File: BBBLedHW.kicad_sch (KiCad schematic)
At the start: 40 parts, among them J3 Barrel_Jack_Switch, Q1 2N7002, U1 STM32WB55CEUx, U2 TPS7A2033DBV, U3 SN74LVC1T45DBV, U4 ADP2303ARDZ-5.0, X1 32MHz, X2 32kHz768

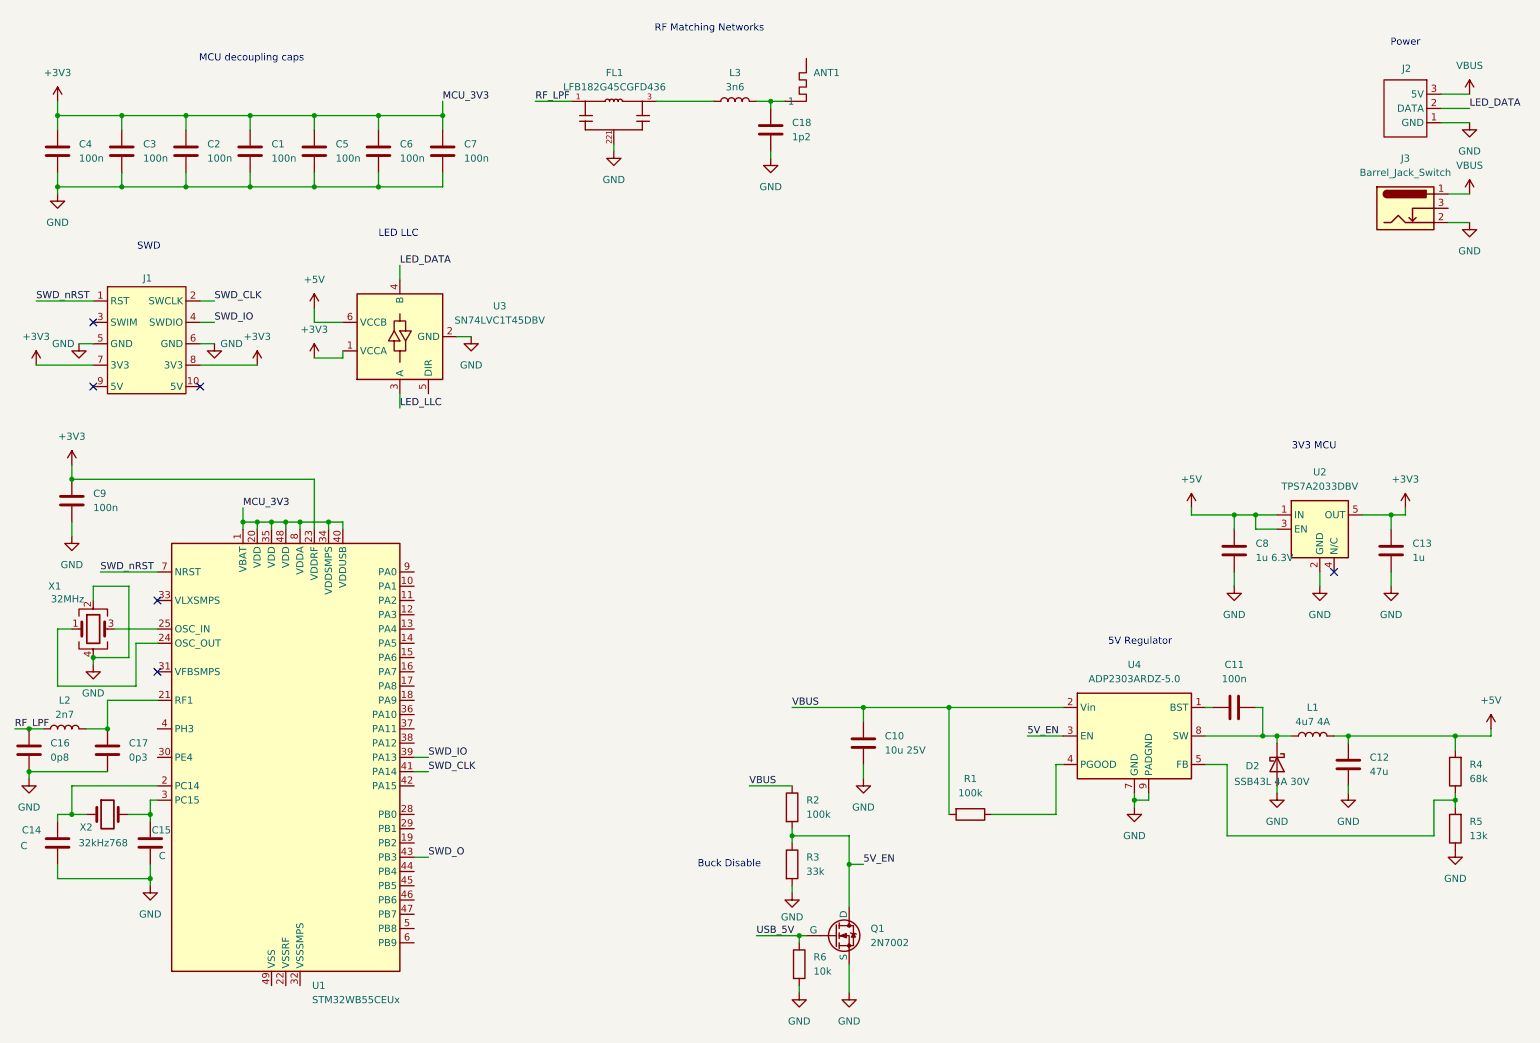
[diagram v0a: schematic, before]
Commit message: Final touches before review
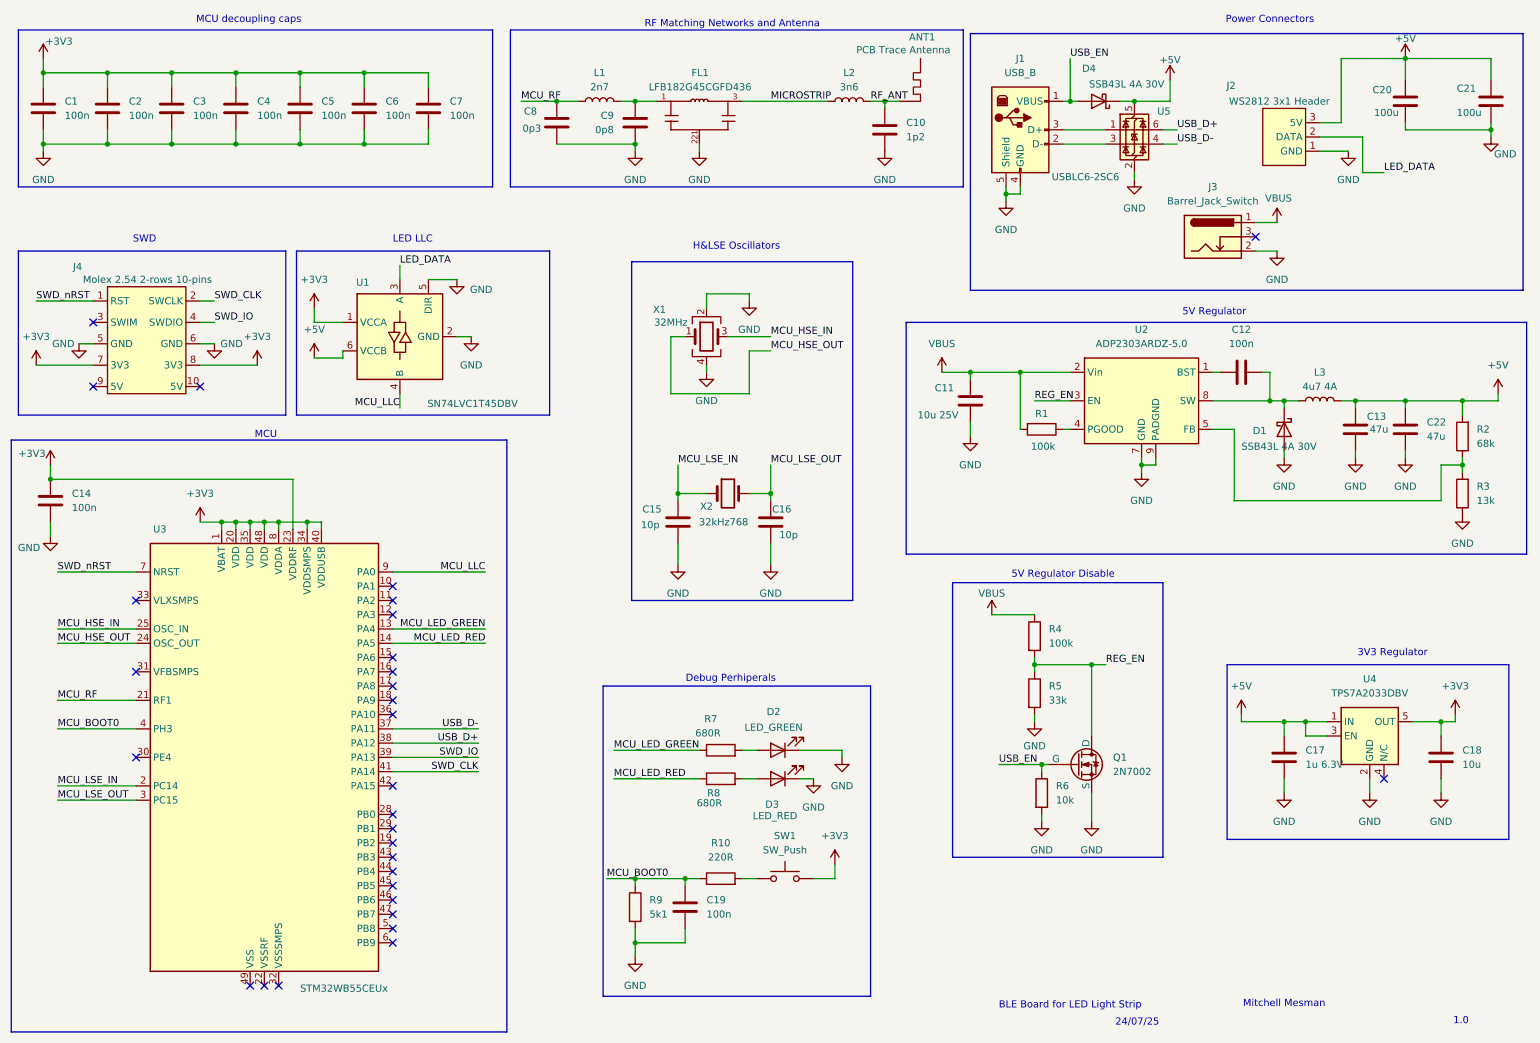
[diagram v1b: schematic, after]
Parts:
- added C19: 100n, symbol Device:C
- added C20, C21: 100u, symbol Device:C
- added C22: 47u, symbol Device:C
- added D2: LED_GREEN, symbol Device:LED
- added D3: LED_RED, symbol Device:LED
- added D4: SSB43L 4A 30V, symbol Device:D_Schottky
- added J1: USB_B, symbol Connector:USB_B
- added R10: 220R, symbol Device:R
- added R7, R8: 680R, symbol Device:R
- added R9: 5k1, symbol Device:R
- added SW1: SW_Push, symbol Switch:SW_Push
- added U5: USBLC6-2SC6, Package_TO_SOT_SMD:SOT-23-6, symbol Power_Protection:USBLC6-2SC6
- ANT1: value ~ -> PCB Trace Antenna
- C15: renamed from C14; value C -> 10p
- C16: renamed from C15; value C -> 10p
- C18: renamed from C13; value 1u -> 10u
- J2: value ~ -> WS2812 3x1 Header
- J4: renamed from J1; value ~ -> Molex 2.54 2-rows 10-pins
- renumbered C4 to C1, C18 to C10, C10 to C11, C11 to C12, C12 to C13, C9 to C14, C8 to C17, C3 to C2, C2 to C3, C1 to C4, C17 to C8, C16 to C9, D2 to D1, L2 to L1, L3 to L2, L1 to L3, R4 to R2, R5 to R3, R2 to R4, R3 to R5, U3 to U1, U4 to U2, U1 to U3, U2 to U4
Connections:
- net LED_LLC is gone; now on net LED_DATA: U1.3 (A)
- net +3V3: now also SW1.2
- net +5V: now also J2.3 (5V), C20.1, C21.1, C22.1, D4.1 (K), U5.5 (VBUS)
- net GND: now also U1.5 (DIR), C19.2, C20.2, C21.2, C22.2, D2.1 (K), D3.1 (K), J1.4 (GND), J1.5 (Shield), R9.2, U5.2 (GND)
- net LED_DATA: no longer U1.4 (B)
- net VBUS: no longer J2.3 (5V)
- net MCU_LSE_OUT: now reaches C16.1, U3.3 (PC15), X2.2
- net MCU_LED_GREEN: now reaches U3.13 (PA4)
- net MCU_LED_GREEN: now also R7.1
- net MCU_LED_RED: now reaches U3.14 (PA5)
- net MCU_LED_RED: now also R8.1
- net MCU_LSE_IN: now reaches C15.1, U3.2 (PC14), X2.1
- net MCU_RF: now reaches C8.1, L1.2, U3.21 (RF1)
- net MCU_HSE_OUT: now reaches U3.24 (OSC_OUT), X1.1
- net MCU_HSE_IN: now reaches U3.25 (OSC_IN), X1.3
- net USB_D-: now reaches U3.37 (PA11)
- net USB_D-: now also U5.4 (I/O2)
- net USB_D+: now reaches U3.38 (PA12)
- net USB_D+: now also U5.6 (I/O1)
- net MCU_BOOT0: now reaches U3.4 (PH3)
- net MCU_BOOT0: now also C19.1, R10.1, R9.1
- net MCU_LLC: now reaches U3.9 (PA0)
- net MCU_LLC: now also U1.4 (B)
- net MICROSTRIP: now reaches FL1.3, L2.1
- net RF_ANT: now reaches ANT1., C10.1, L2.2
- net 5V_EN renamed REG_EN
- net RF_LPF: no longer names the net of C9.1, FL1.1, L1.1
- net SWD_O: no longer names the net of U3.43 (PB3)
- net USB_5V renamed USB_EN
- net USB_EN: now also D4.2 (A), J1.1 (VBUS)
- new net: D2.2 (A), R7.2
- new net: J1.3 (D+), U5.1 (I/O1)
- new net: J1.2 (D-), U5.3 (I/O2)
- new net: D3.2 (A), R8.2
- new net: R10.2, SW1.1
- no-connect marks 6 -> 30
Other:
- note added: "1.0"
- note added: "24/07/25"
- note added: "3V3 Regulator"
- note added: "5V Regulator Disable"
- note added: "BLE Board for LED Light Strip"
- note added: "Debug Perhiperals"
- note added: "H&LSE Oscillators"
- note added: "MCU"
- note added: "Mitchell Mesman"
- note added: "Power Connectors"
- note added: "RF Matching Networks and Antenna"
- note removed: "3V3 MCU"
- note removed: "Buck Disable"
- note removed: "Power"
- note removed: "RF Matching Networks"
- moved on the sheet: C1, C10, C11, C12, C13, C14, C15, C16, C17, C18, C2, C3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

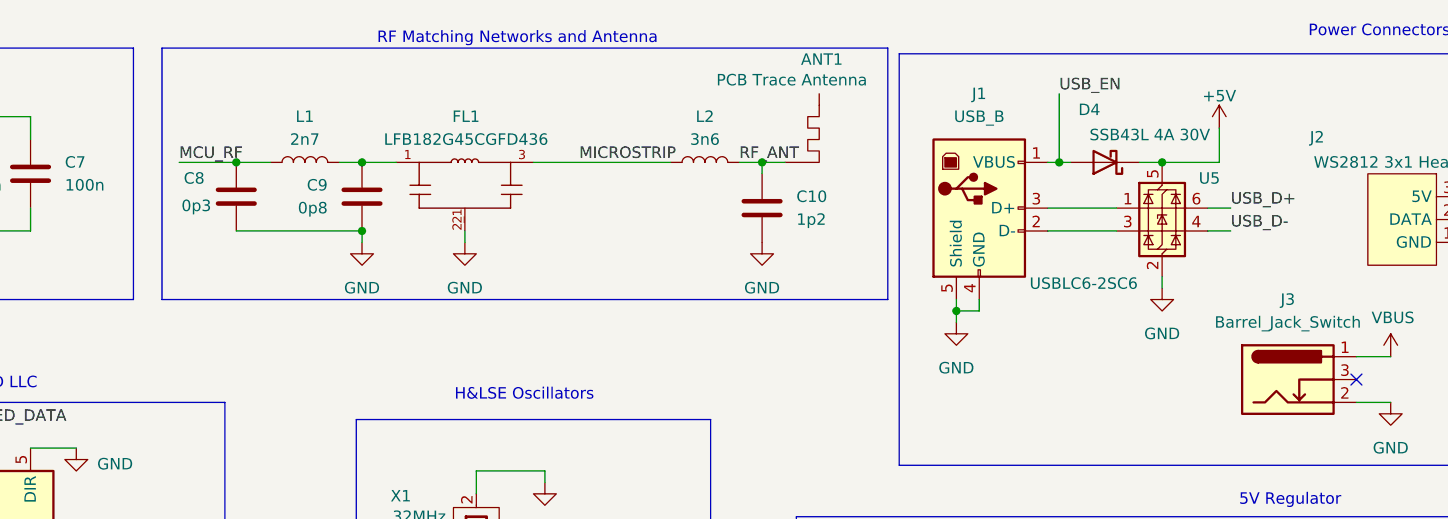
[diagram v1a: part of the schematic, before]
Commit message: Add reviewed schematic
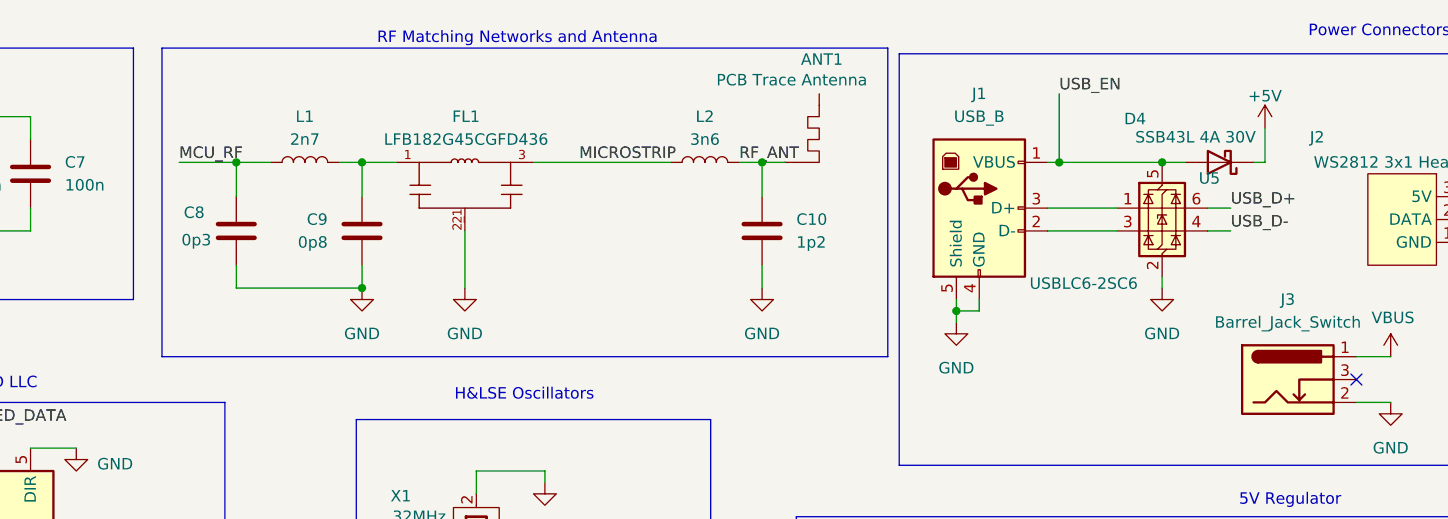
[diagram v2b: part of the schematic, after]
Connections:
- net +5V: no longer U5.5 (VBUS)
- net USB_EN: now also U5.5 (VBUS)
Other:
- moved on the sheet: C10, C8, C9, D4
